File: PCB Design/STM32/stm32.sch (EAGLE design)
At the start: 68 parts, among them IC1 NCP1117ST50T3G, Q1 ABM3B-8.000MHZ-10-1UT, T5 BC847, T6 BC847, T7 BC847, T8 BC847, U1 STM32F103RET6, U2 MCP1700T-3302E/TT, U3 MCP1700T-3302E/TT, U4 MPU-6050, U5 TB6612FNG, X1 22-23-2031

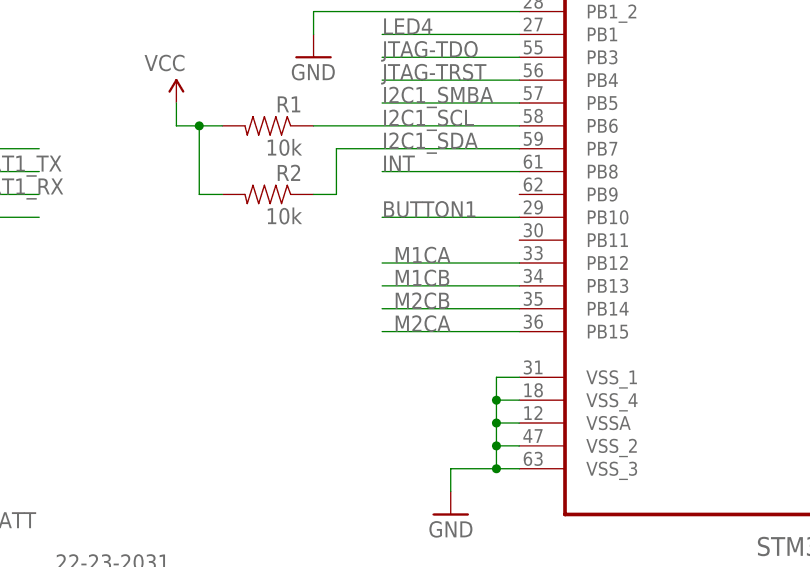
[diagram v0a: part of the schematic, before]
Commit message: save
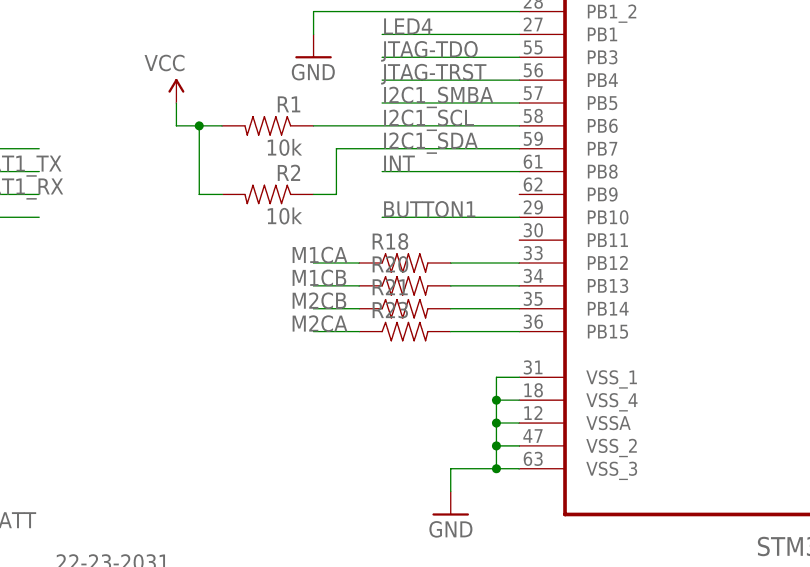
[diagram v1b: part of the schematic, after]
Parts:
- added R18, R20, R21, R23: (no value), SparkFun-Resistors:RESISTOR0805-RES
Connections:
- new net N$20: R18.2, U1.PB12
- new net N$21: R20.2, U1.PB13
- new net N$29: R21.2, U1.PB14
- new net N$30: R23.2, U1.PB15
- net M1CA: now also R18.1; no longer U1.PB12
- net M1CB: now also R20.1; no longer U1.PB13
- net M2CA: now also R23.1; no longer U1.PB15
- net M2CB: now also R21.1; no longer U1.PB14
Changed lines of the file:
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@@
 <part name="SUPPLY19" library="SparkFun-Aesthetics" deviceset="5V" device=""/>
 <part name="SUPPLY23" library="SparkFun-Aesthetics" deviceset="5V" device=""/>
+<part name="R18" library="SparkFun-Resistors" deviceset="RESISTOR" device="0805-RES"/>
+<part name="R20" library="SparkFun-Resistors" deviceset="RESISTOR" device="0805-RES"/>
+<part name="R21" library="SparkFun-Resistors" deviceset="RESISTOR" device="0805-RES"/>
+<part name="R23" library="SparkFun-Resistors" deviceset="RESISTOR" device="0805-RES"/>
 </parts>
 <sheets>
@@
 <instance part="SUPPLY19" gate="G$1" x="429.26" y="134.62"/>
 <instance part="SUPPLY23" gate="G$1" x="429.26" y="114.3"/>
+<instance part="R18" gate="G$1" x="149.86" y="165.1"/>
+<instance part="R20" gate="G$1" x="149.86" y="162.56"/>
+<instance part="R21" gate="G$1" x="149.86" y="160.02"/>
+<instance part="R23" gate="G$1" x="149.86" y="157.48"/>
 </instances>
 <busses>
@@
 <net name="M1CB" class="0">
 <segment>
-<wire x1="162.56" y1="162.56" x2="147.32" y2="162.56" width="0.1524" layer="91"/>
-<label x="154.94" y="162.56" size="1.778" layer="95" rot="MR0"/>
-<pinref part="U1" gate="A" pin="PB13"/>
-</segment>
-<segment>
 <pinref part="JP4" gate="G$1" pin="5"/>
 <wire x1="401.32" y1="109.22" x2="393.7" y2="109.22" width="0.1524" layer="91"/>
 <label x="393.7" y="106.68" size="1.778" layer="95"/>
 </segment>
+<segment>
+<pinref part="R20" gate="G$1" pin="1"/>
+<wire x1="144.78" y1="162.56" x2="139.7" y2="162.56" width="0.1524" layer="91"/>
+<label x="137.16" y="162.56" size="1.778" layer="95"/>
+</segment>
 </net>
 <net name="M1CA" class="0">
-<segment>
-<wire x1="162.56" y1="165.1" x2="147.32" y2="165.1" width="0.1524" layer="91"/>
-<label x="154.94" y="165.1" size="1.778" layer="95" rot="MR0"/>
-<pinref part="U1" gate="A" pin="PB12"/>
-</segment>
 <segment>
 <pinref part="JP4" gate="G$1" pin="6"/>
@@
 <label x="419.1" y="106.68" size="1.778" layer="95"/>
 </segment>
+<segment>
+<pinref part="R18" gate="G$1" pin="1"/>
+<wire x1="144.78" y1="165.1" x2="139.7" y2="165.1" width="0.1524" layer="91"/>
+<label x="137.16" y="165.1" size="1.778" layer="95"/>
+</segment>
 </net>
 <net name="M2CA" class="0">
@@
 </segment>
 <segment>
-<wire x1="162.56" y1="157.48" x2="147.32" y2="157.48" width="0.1524" layer="91"/>
-<label x="154.94" y="157.48" size="1.778" layer="95" rot="MR0"/>
-<pinref part="U1" gate="A" pin="PB15"/>
+<pinref part="R23" gate="G$1" pin="1"/>
+<wire x1="144.78" y1="157.48" x2="139.7" y2="157.48" width="0.1524" layer="91"/>
+<label x="137.16" y="157.48" size="1.778" layer="95"/>
 </segment>
 </net>
@@
 </segment>
 <segment>
-<wire x1="162.56" y1="160.02" x2="147.32" y2="160.02" width="0.1524" layer="91"/>
-<label x="154.94" y="160.02" size="1.778" layer="95" rot="MR0"/>
-<pinref part="U1" gate="A" pin="PB14"/>
+<pinref part="R21" gate="G$1" pin="1"/>
+<wire x1="144.78" y1="160.02" x2="139.7" y2="160.02" width="0.1524" layer="91"/>
+<label x="137.16" y="160.02" size="1.778" layer="95"/>
 </segment>
 </net>
@@
 </segment>
 </net>
+<net name="N$20" class="0">
+<segment>
+<pinref part="R18" gate="G$1" pin="2"/>
+<pinref part="U1" gate="A" pin="PB12"/>
+<wire x1="154.94" y1="165.1" x2="162.56" y2="165.1" width="0.1524" layer="91"/>
+</segment>
+</net>
+<net name="N$21" class="0">
+<segment>
+<pinref part="R20" gate="G$1" pin="2"/>
+<pinref part="U1" gate="A" pin="PB13"/>
+<wire x1="154.94" y1="162.56" x2="162.56" y2="162.56" width="0.1524" layer="91"/>
+</segment>
+</net>
+<net name="N$29" class="0">
+<segment>
+<pinref part="R21" gate="G$1" pin="2"/>
+<pinref part="U1" gate="A" pin="PB14"/>
+<wire x1="154.94" y1="160.02" x2="162.56" y2="160.02" width="0.1524" layer="91"/>
+</segment>
+</net>
+<net name="N$30" class="0">
+<segment>
+<pinref part="R23" gate="G$1" pin="2"/>
+<pinref part="U1" gate="A" pin="PB15"/>
+<wire x1="154.94" y1="157.48" x2="162.56" y2="157.48" width="0.1524" layer="91"/>
+</segment>
+</net>

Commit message: sleep
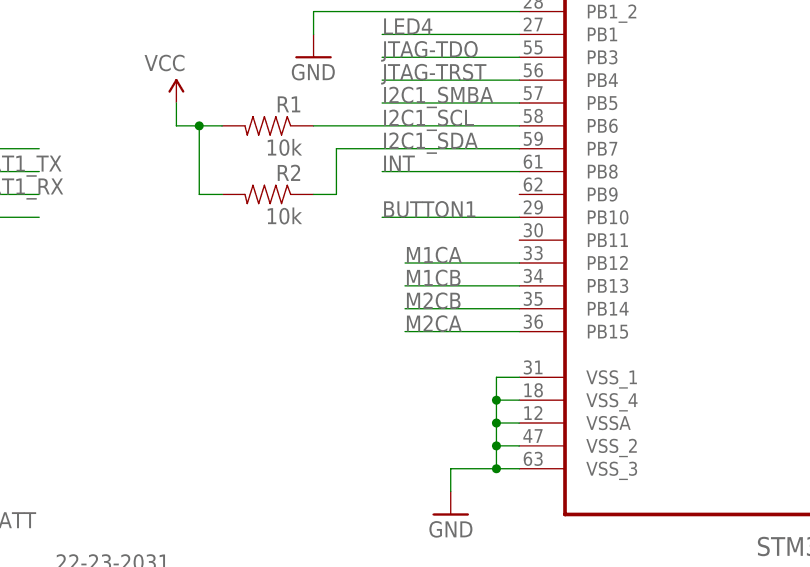
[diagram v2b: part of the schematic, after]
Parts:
- removed R18, R20, R21, R23: (no value), SparkFun-Resistors:RESISTOR0805-RES
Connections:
- removed net N$20: R18.2, U1.PB12
- removed net N$21: R20.2, U1.PB13
- removed net N$29: R21.2, U1.PB14
- removed net N$30: R23.2, U1.PB15
- net M1CA: now also U1.PB12; no longer R18.1
- net M1CB: now also U1.PB13; no longer R20.1
- net M2CA: now also U1.PB15; no longer R23.1
- net M2CB: now also U1.PB14; no longer R21.1
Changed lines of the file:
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@@
 <part name="SUPPLY19" library="SparkFun-Aesthetics" deviceset="5V" device=""/>
 <part name="SUPPLY23" library="SparkFun-Aesthetics" deviceset="5V" device=""/>
-<part name="R18" library="SparkFun-Resistors" deviceset="RESISTOR" device="0805-RES"/>
-<part name="R20" library="SparkFun-Resistors" deviceset="RESISTOR" device="0805-RES"/>
-<part name="R21" library="SparkFun-Resistors" deviceset="RESISTOR" device="0805-RES"/>
-<part name="R23" library="SparkFun-Resistors" deviceset="RESISTOR" device="0805-RES"/>
 </parts>
 <sheets>
@@
 <instance part="SUPPLY19" gate="G$1" x="429.26" y="134.62"/>
 <instance part="SUPPLY23" gate="G$1" x="429.26" y="114.3"/>
-<instance part="R18" gate="G$1" x="149.86" y="165.1"/>
-<instance part="R20" gate="G$1" x="149.86" y="162.56"/>
-<instance part="R21" gate="G$1" x="149.86" y="160.02"/>
-<instance part="R23" gate="G$1" x="149.86" y="157.48"/>
 </instances>
 <busses>
@@
 </segment>
 <segment>
-<pinref part="R20" gate="G$1" pin="1"/>
-<wire x1="144.78" y1="162.56" x2="139.7" y2="162.56" width="0.1524" layer="91"/>
-<label x="137.16" y="162.56" size="1.778" layer="95"/>
+<wire x1="162.56" y1="162.56" x2="149.86" y2="162.56" width="0.1524" layer="91"/>
+<label x="149.86" y="162.56" size="1.778" layer="95"/>
+<pinref part="U1" gate="A" pin="PB13"/>
 </segment>
 </net>
@@
 </segment>
 <segment>
-<pinref part="R18" gate="G$1" pin="1"/>
-<wire x1="144.78" y1="165.1" x2="139.7" y2="165.1" width="0.1524" layer="91"/>
-<label x="137.16" y="165.1" size="1.778" layer="95"/>
+<wire x1="162.56" y1="165.1" x2="149.86" y2="165.1" width="0.1524" layer="91"/>
+<label x="149.86" y="165.1" size="1.778" layer="95"/>
+<pinref part="U1" gate="A" pin="PB12"/>
 </segment>
 </net>
@@
 </segment>
 <segment>
-<pinref part="R23" gate="G$1" pin="1"/>
-<wire x1="144.78" y1="157.48" x2="139.7" y2="157.48" width="0.1524" layer="91"/>
-<label x="137.16" y="157.48" size="1.778" layer="95"/>
+<wire x1="162.56" y1="157.48" x2="149.86" y2="157.48" width="0.1524" layer="91"/>
+<label x="149.86" y="157.48" size="1.778" layer="95"/>
+<pinref part="U1" gate="A" pin="PB15"/>
 </segment>
 </net>
@@
 </segment>
 <segment>
-<pinref part="R21" gate="G$1" pin="1"/>
-<wire x1="144.78" y1="160.02" x2="139.7" y2="160.02" width="0.1524" layer="91"/>
-<label x="137.16" y="160.02" size="1.778" layer="95"/>
+<wire x1="162.56" y1="160.02" x2="149.86" y2="160.02" width="0.1524" layer="91"/>
+<label x="149.86" y="160.02" size="1.778" layer="95"/>
+<pinref part="U1" gate="A" pin="PB14"/>
 </segment>
 </net>
@@
 </segment>
 </net>
-<net name="N$20" class="0">
-<segment>
-<pinref part="R18" gate="G$1" pin="2"/>
-<pinref part="U1" gate="A" pin="PB12"/>
-<wire x1="154.94" y1="165.1" x2="162.56" y2="165.1" width="0.1524" layer="91"/>
-</segment>
-</net>
-<net name="N$21" class="0">
-<segment>
-<pinref part="R20" gate="G$1" pin="2"/>
-<pinref part="U1" gate="A" pin="PB13"/>
-<wire x1="154.94" y1="162.56" x2="162.56" y2="162.56" width="0.1524" layer="91"/>
-</segment>
-</net>
-<net name="N$29" class="0">
-<segment>
-<pinref part="R21" gate="G$1" pin="2"/>
-<pinref part="U1" gate="A" pin="PB14"/>
-<wire x1="154.94" y1="160.02" x2="162.56" y2="160.02" width="0.1524" layer="91"/>
-</segment>
-</net>
-<net name="N$30" class="0">
-<segment>
-<pinref part="R23" gate="G$1" pin="2"/>
-<pinref part="U1" gate="A" pin="PB15"/>
-<wire x1="154.94" y1="157.48" x2="162.56" y2="157.48" width="0.1524" layer="91"/>
-</segment>
-</net>
